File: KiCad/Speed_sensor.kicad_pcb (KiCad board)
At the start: 2 copper layers, 70 parts, among them J1 USB_B_Micro, J2 SWD, U1 BQ24040DSQR, U2 TP1941U, U3 ST1PS02, U4 nRF52832-QFxx, U5 LIS2DH12, Y1 32,768kHz, Y2 32MHz

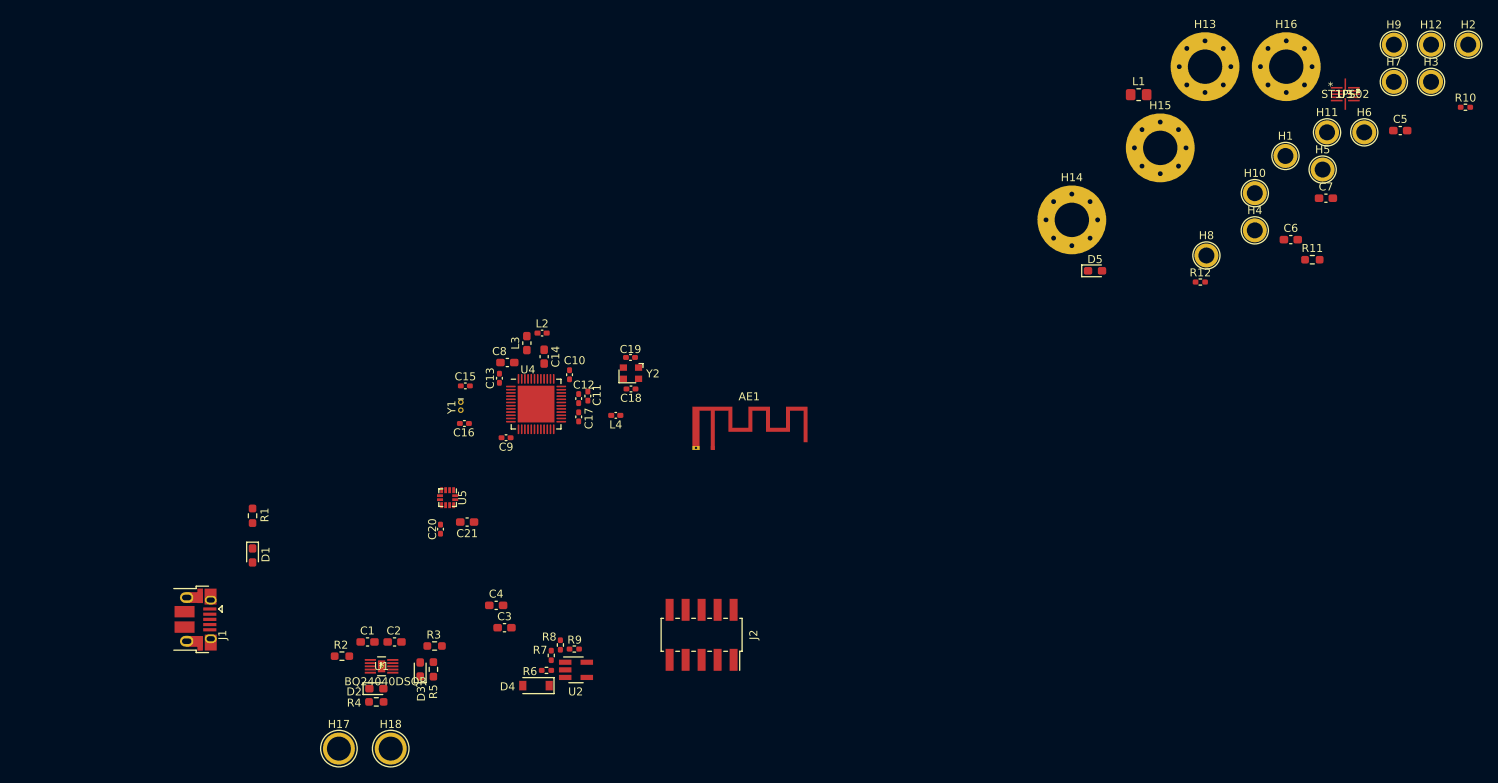
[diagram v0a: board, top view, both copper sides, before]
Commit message: layout. parts roughly put into the right spot
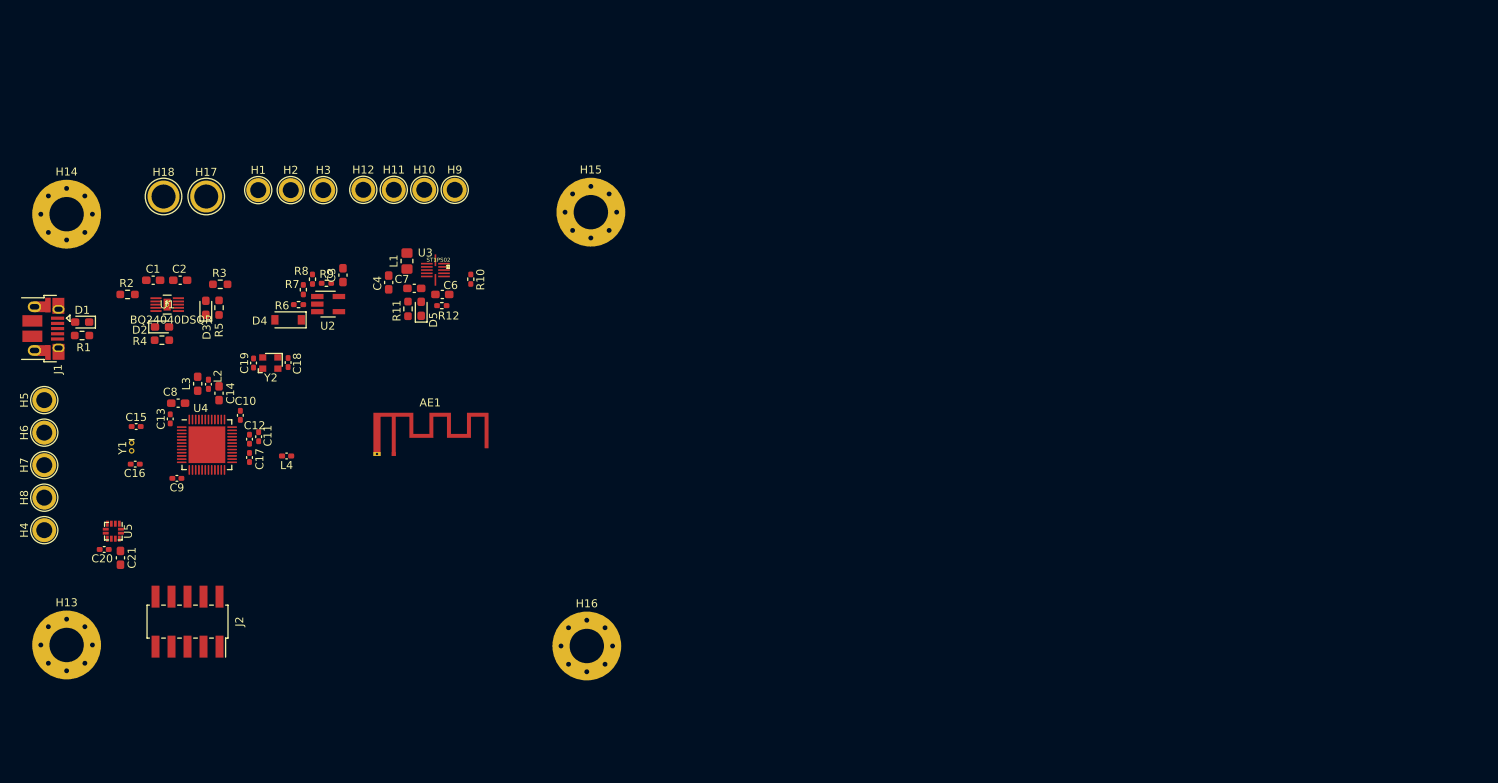
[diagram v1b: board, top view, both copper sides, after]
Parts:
- removed the C3 at (154.3, 92.2)
- moved H7 175.4 mm to (96.8, 71.9), turned to 90 degrees
- moved H6 169.2 mm to (96.8, 67.8), turned to 90 degrees
- moved H5 162.4 mm to (96.8, 63.8), turned to 90 degrees
- moved H13 159.6 mm to (99.6, 94.4)
- moved H4 155.9 mm to (96.8, 80.0), turned to 90 degrees
- moved H8 148.4 mm to (96.8, 75.9), turned to 90 degrees
- moved H2 148.3 mm to (127.6, 37.5)
- moved H3 139.1 mm to (131.6, 37.5)
- moved H12 134.7 mm to (136.7, 37.5)
- moved H1 128.5 mm to (123.5, 37.5)
- moved C4 127.9 mm to (139.8, 49.0), turned to 270 degrees
- moved R10 126.2 mm to (150.1, 48.6), turned to 270 degrees
- moved H14 125.7 mm to (99.6, 40.5)
- moved H9 118.8 mm to (148.1, 37.5)
- moved H11 116.9 mm to (140.5, 37.5)
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- renumbered C4 to C3, C5 to C4

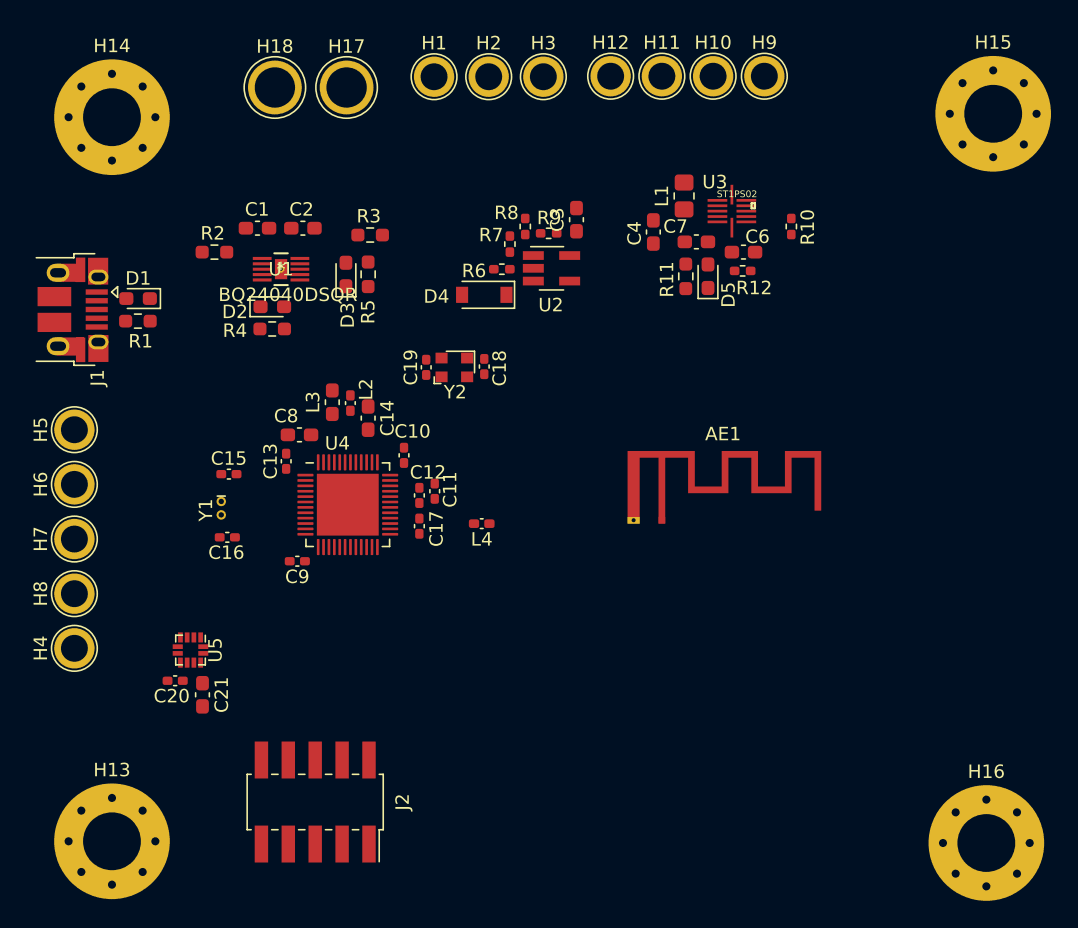
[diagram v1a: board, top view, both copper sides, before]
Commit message: played around with part positioning slightly
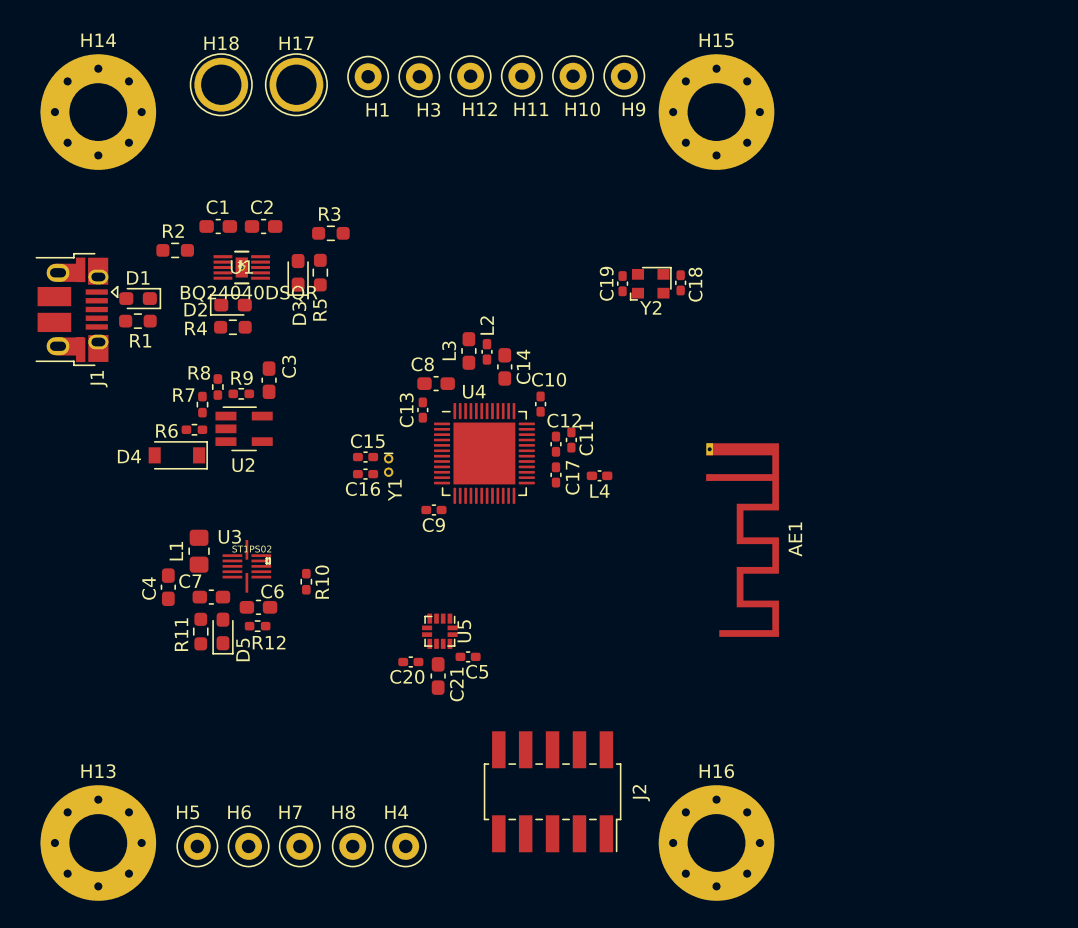
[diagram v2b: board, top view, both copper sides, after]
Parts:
- removed H2: Vout2, TestPoint:TestPoint_Plated_Hole_D2.0mm
- added C5: 100n, Capacitor_SMD:C_0402_1005Metric_Pad0.74x0.62mm_HandSolder, F.Cu at (126.1, 80.6)
- AE1: value Antenna -> 2,4GHz
- H1, H10, H11, H12, H3, H4, H5, H6, H7, H8, H9: footprint TestPoint:TestPoint_Plated_Hole_D2.0mm -> TestPoint:TestPoint_Loop_D1.80mm_Drill1.0mm_Beaded
- moved C7 44.7 mm to (107.0, 76.2)
- moved R10 44.7 mm to (114.0, 75.1)
- moved R11 44.7 mm to (106.2, 78.8)
- moved R12 44.7 mm to (110.4, 78.4)
- moved U3 44.7 mm to (109.6, 73.9)
- moved C4 44.7 mm to (103.8, 75.5)
- moved C6 44.7 mm to (110.5, 77.0)
- moved D5 44.7 mm to (107.8, 78.8)
- moved L1 44.7 mm to (106.0, 72.8)
- moved H5 32.3 mm to (105.9, 94.7), turned to 180 degrees
- moved H6 29.9 mm to (109.7, 94.7), turned to 180 degrees
- moved H4 28.7 mm to (121.4, 94.7), turned to 180 degrees
- moved H7 28.3 mm to (113.5, 94.7), turned to 180 degrees
- moved H8 28.0 mm to (117.5, 94.7), turned to 180 degrees
- moved D4 25.8 mm to (104.4, 65.7)
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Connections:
- AE1 pad 2: (no net) -> BQ_VSS
